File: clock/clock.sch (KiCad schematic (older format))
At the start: 166 parts, among them J1 Conn_02x05_Odd_Even, P1 Conn_WallPlug, T1 120 to 12, U1 74HC596, U10 74HC596, U11 PIC18F45K20_44-PIN_TQFP, U2 74HC596, U3 74HC596, U4 74HC596, U5 74HC596, U6 74HC596, U7 L78L33ABU, U8 74HC596, U9 74HC596

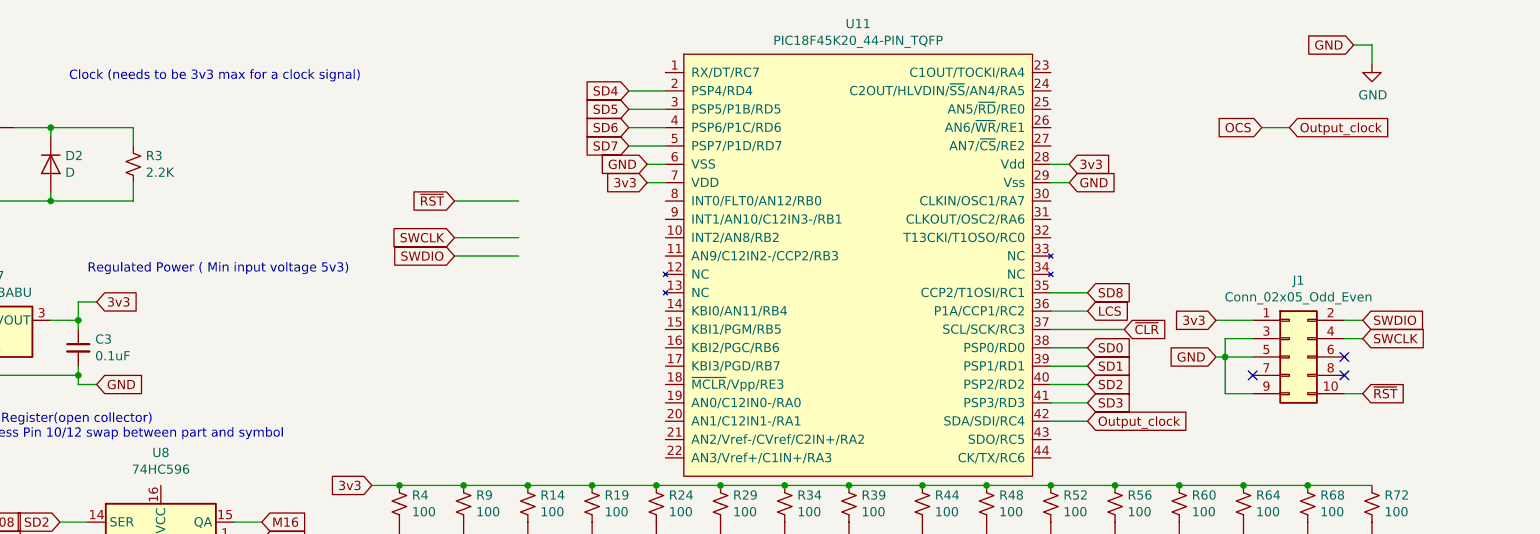
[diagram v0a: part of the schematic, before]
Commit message: Updated todo list and some tracing
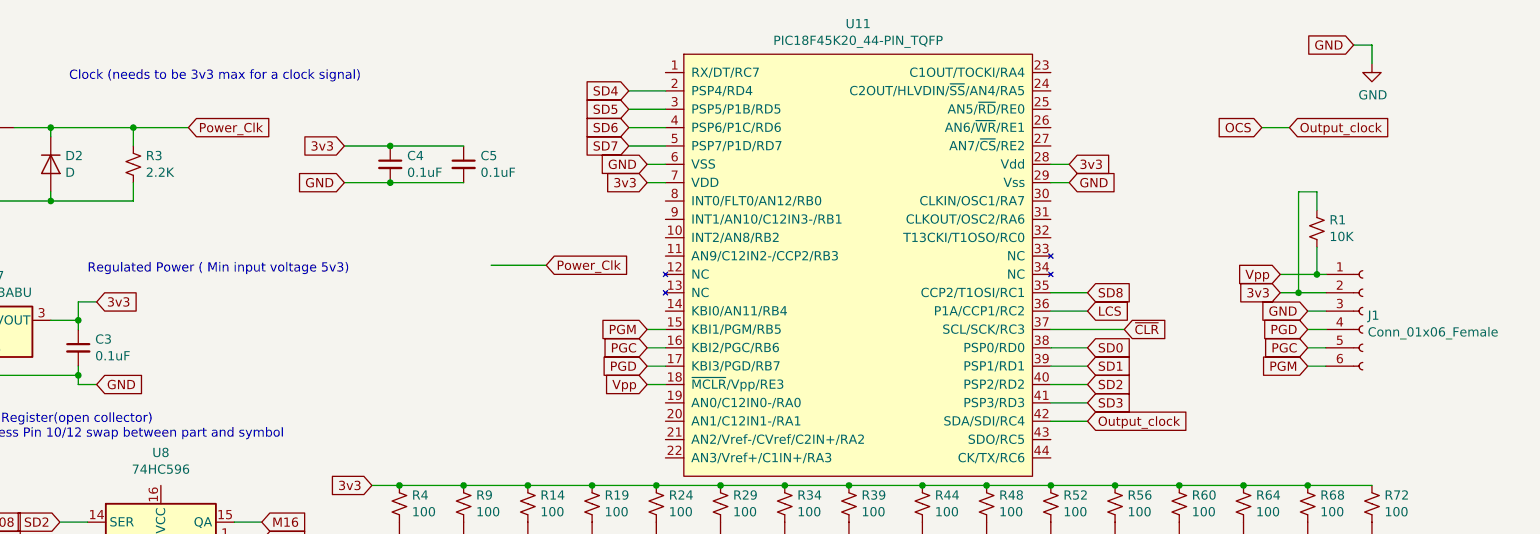
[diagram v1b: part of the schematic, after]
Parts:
- removed J1: Conn_02x05_Odd_Even, Connector_PinHeader_1.27mm:PinHeader_2x05_P1.27mm_Vertical, symbol Connector_Generic:Conn_02x05_Odd_Even
- added C4, C5: 0.1uF, Capacitor_SMD:C_0805_2012Metric, symbol Device:C_Small
- added J1: Conn_01x06_Female, Connector_PinHeader_2.54mm:PinHeader_1x06_P2.54mm_Vertical, symbol Connector:Conn_01x06_Female
- added R1: 10K, Resistor_SMD:R_0805_2012Metric, symbol Device:R_Small_US
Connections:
- net 3v3: now also C4.1, C5.1, J1.2 (Pin_2), R1.1
- net GND: now also C4.2, C5.2, J1.3 (Pin_3)
- net Power_Clk: now reaches D2.1 (K), D75.1 (K), R3.2
- net PGM: now reaches U11.15 (KBI1/PGM/RB5)
- net PGM: now also J1.6 (Pin_6)
- net PGC: now reaches U11.16 (KBI2/PGC/RB6)
- net PGC: now also J1.5 (Pin_5)
- net PGD: now reaches U11.17 (KBI3/PGD/RB7)
- net PGD: now also J1.4 (Pin_4)
- net Vpp: now reaches U11.18 (~MCLR~/Vpp/RE3)
- net Vpp: now also J1.1 (Pin_1), R1.2
- no-connect marks 3 -> 0
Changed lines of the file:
@@
 Wire Wire Line
 	7000 1250 7100 1250
-$Comp
-L Connector_Generic:Conn_02x05_Odd_Even J1
-U 1 1 5E00183C
-P 10500 2300
-F 0 "J1" H 10550 2717 50  0000 C CNN
-F 1 "Conn_02x05_Odd_Even" H 10550 2626 50  0000 C CNN
-F 2 "Connector_PinHeader_1.27mm:PinHeader_2x05_P1.27mm_Vertical" H 10500 2300 50  0001 C CNN
-F 3 "~" H 10500 2300 50  0001 C CNN
-	1    10500 2300
-	1    0    0    -1
-$EndComp
-Text GLabel 10100 2100 0    50   Input ~ 0
-3v3
-Wire Wire Line
-	10100 2100 10300 2100
-Text GLabel 10100 2300 0    50   Input ~ 0
-GND
-Wire Wire Line
-	10300 2200 10150 2200
-Wire Wire Line
-	10150 2200 10150 2300
-Wire Wire Line
-	10150 2300 10100 2300
-Wire Wire Line
-	10300 2300 10150 2300
-Connection ~ 10150 2300
-Wire Wire Line
-	10300 2500 10150 2500
-Wire Wire Line
-	10150 2500 10150 2300
-NoConn ~ 10300 2400
-NoConn ~ 10800 2400
-NoConn ~ 10800 2300
-Text GLabel 10900 2500 2    50   Input ~ 0
-~RST
-Text GLabel 10900 2200 2    50   Input ~ 0
-SWCLK
-Text GLabel 10900 2100 2    50   Input ~ 0
-SWDIO
-Wire Wire Line
-	10800 2100 10900 2100
-Wire Wire Line
-	10800 2200 10900 2200
-Wire Wire Line
-	10800 2500 10900 2500
-Text GLabel 5950 1750 0    50   Input ~ 0
-SWDIO
-Text GLabel 5950 1650 0    50   Input ~ 0
-SWCLK
-Wire Wire Line
-	5950 1650 6300 1650
-Wire Wire Line
-	5950 1750 6300 1750
-Text GLabel 5950 1450 0    50   Input ~ 0
-~RST
-Wire Wire Line
-	5950 1450 6300 1450
 Text GLabel 7000 1350 0    50   Input ~ 0
 3v3
@@
 Wire Wire Line
 	9300 1250 9200 1250
+$Comp
+L Connector:Conn_01x06_Female J1
+U 1 1 5F0042BD
+P 10900 2050
+F 0 "J1" H 10927 2026 50  0000 L CNN
+F 1 "Conn_01x06_Female" H 10927 1935 50  0000 L CNN
+F 2 "Connector_PinHeader_2.54mm:PinHeader_1x06_P2.54mm_Vertical" H 10900 2050 50  0001 C CNN
+F 3 "~" H 10900 2050 50  0001 C CNN
+	1    10900 2050
+	1    0    0    -1
+$EndComp
+Text GLabel 10600 2050 0    50   Input ~ 0
+GND
+Wire Wire Line
+	10600 2050 10700 2050
+Text GLabel 10450 1950 0    50   Input ~ 0
+3v3
+Wire Wire Line
+	10450 1950 10550 1950
+Text GLabel 7000 2150 0    50   Input ~ 0
+PGM
+Wire Wire Line
+	7000 2150 7100 2150
+Text GLabel 7000 2250 0    50   Input ~ 0
+PGC
+Wire Wire Line
+	7000 2250 7100 2250
+Text GLabel 7000 2350 0    50   Input ~ 0
+PGD
+Wire Wire Line
+	7000 2350 7100 2350
+Text GLabel 7000 2450 0    50   Input ~ 0
+Vpp
+Wire Wire Line
+	7000 2450 7100 2450
+Text GLabel 10450 1850 0    50   Input ~ 0
+Vpp
+Wire Wire Line
+	10450 1850 10650 1850
+Text GLabel 10600 2350 0    50   Input ~ 0
+PGM
+Wire Wire Line
+	10600 2350 10700 2350
+Text GLabel 10600 2250 0    50   Input ~ 0
+PGC
+Wire Wire Line
+	10600 2250 10700 2250
+Text GLabel 10600 2150 0    50   Input ~ 0
+PGD
+Wire Wire Line
+	10600 2150 10700 2150
+$Comp
+L Device:R_Small_US R1
+U 1 1 5F3D672D
+P 10650 1600
+F 0 "R1" H 10718 1646 50  0000 L CNN
+F 1 "10K" H 10718 1555 50  0000 L CNN
+F 2 "Resistor_SMD:R_0805_2012Metric" H 10650 1600 50  0001 C CNN
+F 3 "~" H 10650 1600 50  0001 C CNN
+	1    10650 1600
+	1    0    0    -1
+$EndComp
+Wire Wire Line
+	10650 1700 10650 1850
+Connection ~ 10650 1850
+Wire Wire Line
+	10650 1850 10700 1850
+Wire Wire Line
+	10650 1500 10650 1400
+Wire Wire Line
+	10650 1400 10550 1400
+Wire Wire Line
+	10550 1400 10550 1950
+Connection ~ 10550 1950
+Wire Wire Line
+	10550 1950 10700 1950
+$Comp
+L Device:C_Small C4
+U 1 1 5F53ABE7
+P 5600 1250
+F 0 "C4" H 5692 1296 50  0000 L CNN
+F 1 "0.1uF" H 5692 1205 50  0000 L CNN
+F 2 "Capacitor_SMD:C_0805_2012Metric" H 5600 1250 50  0001 C CNN
+F 3 "~" H 5600 1250 50  0001 C CNN
+	1    5600 1250
+	1    0    0    -1
+$EndComp
+$Comp
+L Device:C_Small C5
+U 1 1 5F53B196
+P 6000 1250
+F 0 "C5" H 6092 1296 50  0000 L CNN
+F 1 "0.1uF" H 6092 1205 50  0000 L CNN
+F 2 "Capacitor_SMD:C_0805_2012Metric" H 6000 1250 50  0001 C CNN
+F 3 "~" H 6000 1250 50  0001 C CNN
+	1    6000 1250
+	1    0    0    -1
+$EndComp
+Text GLabel 5350 1350 0    50   Input ~ 0
+GND
+Text GLabel 5350 1150 0    50   Input ~ 0
+3v3
+Wire Wire Line
+	5350 1350 5600 1350
+Connection ~ 5600 1350
+Wire Wire Line
+	5600 1350 6000 1350
+Wire Wire Line
+	5350 1150 5600 1150
+Connection ~ 5600 1150
+Wire Wire Line
+	5600 1150 6000 1150
+Text GLabel 4500 1050 2    50   Input ~ 0
+Power_Clk
+Wire Wire Line
+	4200 1050 4500 1050
+Connection ~ 4200 1050
+Text GLabel 6450 1800 2    50   Input ~ 0
+Power_Clk
+Wire Wire Line
+	6150 1800 6450 1800
 $EndSCHEMATC
